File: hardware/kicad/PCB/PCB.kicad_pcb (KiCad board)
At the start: 2 copper layers, 19 parts, among them J1 USB_C_Receptacle_PowerOnly_6P, J2 Conn_01x05_Socket, J3 Conn_01x02, U1 STM32G030F6Px, U2 MCP73831-2-OT, U3 DW01A, U4 FS8205A_C2830320

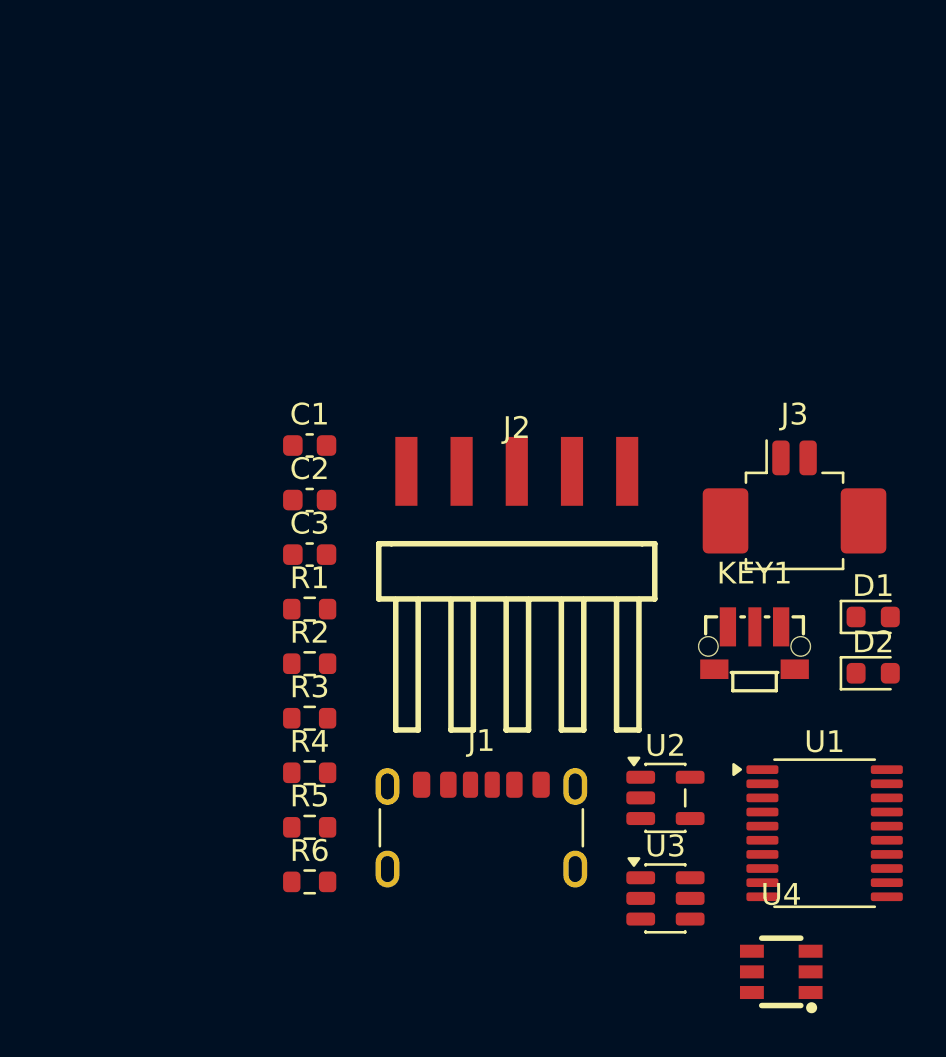
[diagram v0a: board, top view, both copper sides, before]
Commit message: updated PCB design
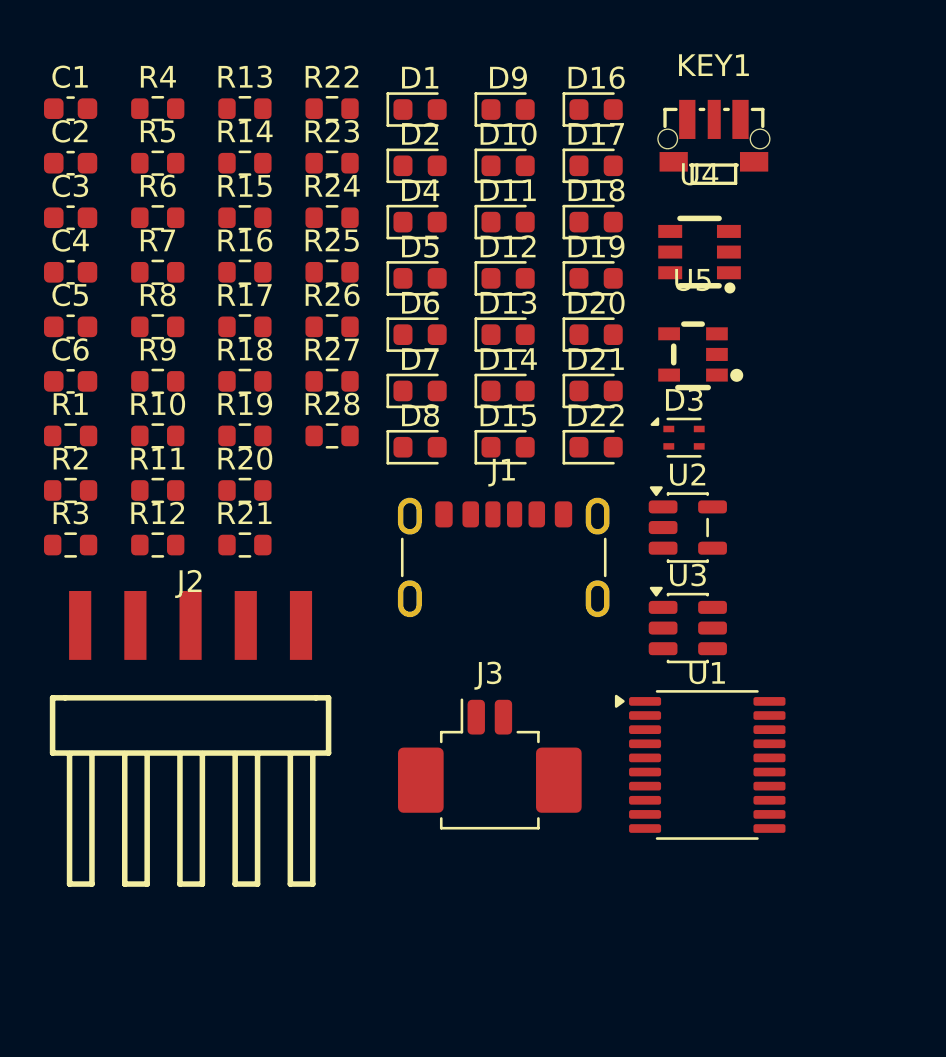
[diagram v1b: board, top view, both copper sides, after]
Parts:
- added C4: 1uF, Capacitor_SMD:C_0603_1608Metric, F.Cu at (18.0, 23.8)
- added C5: 1uF, Capacitor_SMD:C_0603_1608Metric, F.Cu at (18.0, 26.3)
- added C6: 100nF, Capacitor_SMD:C_0603_1608Metric, F.Cu at (18.0, 28.8)
- added D10: LED, Diode_SMD:D_0603_1608Metric, F.Cu at (38.1, 18.9)
- added D11: LED, Diode_SMD:D_0603_1608Metric, F.Cu at (38.1, 21.5)
- added D12: LED, Diode_SMD:D_0603_1608Metric, F.Cu at (38.1, 24.1)
- added D13: LED, Diode_SMD:D_0603_1608Metric, F.Cu at (38.1, 26.7)
- added D14: LED, Diode_SMD:D_0603_1608Metric, F.Cu at (38.1, 29.2)
- added D15: LED, Diode_SMD:D_0603_1608Metric, F.Cu at (38.1, 31.8)
- added D16: LED, Diode_SMD:D_0603_1608Metric, F.Cu at (42.2, 16.3)
- added D17: LED, Diode_SMD:D_0603_1608Metric, F.Cu at (42.2, 18.9)
- added D18: LED, Diode_SMD:D_0603_1608Metric, F.Cu at (42.2, 21.5)
- added D19: LED, Diode_SMD:D_0603_1608Metric, F.Cu at (42.2, 24.1)
- added D20: LED, Diode_SMD:D_0603_1608Metric, F.Cu at (42.2, 26.7)
- added D21: LED, Diode_SMD:D_0603_1608Metric, F.Cu at (42.2, 29.2)
- added D22: LED, Diode_SMD:D_0603_1608Metric, F.Cu at (42.2, 31.8)
- added D3: D_Schottky, Sensor_Humidity:Sensirion_DFN-4_1.5x1.5mm_P0.8mm_SHT4x_NoCentralPad, F.Cu at (46.2, 31.4)
- added D4: LED, Diode_SMD:D_0603_1608Metric, F.Cu at (34.1, 21.5)
- added D5: LED, Diode_SMD:D_0603_1608Metric, F.Cu at (34.1, 24.1)
- added D6: LED, Diode_SMD:D_0603_1608Metric, F.Cu at (34.1, 26.7)
- added D7: LED, Diode_SMD:D_0603_1608Metric, F.Cu at (34.1, 29.2)
- added D8: LED, Diode_SMD:D_0603_1608Metric, F.Cu at (34.1, 31.8)
- added D9: LED, Diode_SMD:D_0603_1608Metric, F.Cu at (38.1, 16.3)
- added R10: 470, Resistor_SMD:R_0603_1608Metric, F.Cu at (22.0, 31.3)
- added R11: 470, Resistor_SMD:R_0603_1608Metric, F.Cu at (22.0, 33.8)
- added R12: 470, Resistor_SMD:R_0603_1608Metric, F.Cu at (22.0, 36.3)
- added R13: 470, Resistor_SMD:R_0603_1608Metric, F.Cu at (26.0, 16.3)
- added R14: 470, Resistor_SMD:R_0603_1608Metric, F.Cu at (26.0, 18.8)
- added R15: 470, Resistor_SMD:R_0603_1608Metric, F.Cu at (26.0, 21.3)
- added R16: 470, Resistor_SMD:R_0603_1608Metric, F.Cu at (26.0, 23.8)
- added R17: 470, Resistor_SMD:R_0603_1608Metric, F.Cu at (26.0, 26.3)
- added R18: 470, Resistor_SMD:R_0603_1608Metric, F.Cu at (26.0, 28.8)
- added R19: 470, Resistor_SMD:R_0603_1608Metric, F.Cu at (26.0, 31.3)
- added R20: 470, Resistor_SMD:R_0603_1608Metric, F.Cu at (26.0, 33.8)
- added R21: 470, Resistor_SMD:R_0603_1608Metric, F.Cu at (26.0, 36.3)
- added R22: 470, Resistor_SMD:R_0603_1608Metric, F.Cu at (30.0, 16.3)
- added R23: 470, Resistor_SMD:R_0603_1608Metric, F.Cu at (30.0, 18.8)
- added R24: 470, Resistor_SMD:R_0603_1608Metric, F.Cu at (30.0, 21.3)
- added R25: 470, Resistor_SMD:R_0603_1608Metric, F.Cu at (30.0, 23.8)
- added R26: 470, Resistor_SMD:R_0603_1608Metric, F.Cu at (30.0, 26.3)
- added R27: 1M, Resistor_SMD:R_0603_1608Metric, F.Cu at (30.0, 28.8)
- added R28: 1M, Resistor_SMD:R_0603_1608Metric, F.Cu at (30.0, 31.3)
- added R7: 470, Resistor_SMD:R_0603_1608Metric, F.Cu at (22.0, 23.8)
- added R8: 470, Resistor_SMD:R_0603_1608Metric, F.Cu at (22.0, 26.3)
- added R9: 470, Resistor_SMD:R_0603_1608Metric, F.Cu at (22.0, 28.8)
- added U5: TPS7A0233PDBVR, JLC2KiCad:SOT-23-5_L2.9-W1.6-P0.95-LS2.8-BR, F.Cu at (46.6, 27.6)
- moved U4 33.3 mm to (46.9, 22.9)
- moved R5 31.3 mm to (22.0, 18.8)
- moved R6 31.3 mm to (22.0, 21.3)
- moved R4 31.3 mm to (22.0, 16.3)
- moved D1 31.3 mm to (34.1, 16.3)
- moved D2 31.3 mm to (34.1, 18.9)
- moved KEY1 23.4 mm to (47.6, 17.7)
- moved C1 19.0 mm to (18.0, 16.3)
- moved C2 19.0 mm to (18.0, 18.8)
- moved C3 19.0 mm to (18.0, 21.3)
- moved J3 18.4 mm to (37.3, 46.7)
- moved J2 16.6 mm to (23.5, 40.0)
- moved R2 13.6 mm to (18.0, 33.8)
- moved R3 13.6 mm to (18.0, 36.3)
- moved R1 13.6 mm to (18.0, 31.3)
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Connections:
- D2 pad 1: unconnected-(D2-K-Pad1) -> TIM14_CH1
- D2 pad 2: unconnected-(D2-A-Pad2) -> Net-(D2-A)
- J2 pad 1: unconnected-(J2-Pin_1-Pad1) -> Net-(D3-A)
- U1 pad 1: unconnected-(U1-PB7/PB8-Pad1) -> TIM16_CH1
- U1 pad 11: unconnected-(U1-PA4-Pad11) -> TIM14_CH1
- U1 pad 13: unconnected-(U1-PA6-Pad13) -> TIM3_CH1
- U1 pad 14: unconnected-(U1-PA7-Pad14) -> TIM3_CH2
- U1 pad 15: unconnected-(U1-PA8/PB0/PB1/PB2-Pad15) -> TIM1_CH2N
- U1 pad 16: unconnected-(U1-PA9/PA11-Pad16) -> TIM1_CH4
- U1 pad 20: unconnected-(U1-PB3/PB4/PB5/PB6-Pad20) -> TIM1_CH3
- U1 pad 4: unconnected-(U1-VDD-Pad4) -> PROG_PWR
- U1 pad 8: unconnected-(U1-PA1-Pad8) -> PA1
